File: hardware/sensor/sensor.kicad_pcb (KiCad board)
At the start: 2 copper layers, 29 x 31 mm, 56 parts, among them P1 CONN_01X05, SW1 Reset, T1 BUK9Y22, U1 LMR16006, U2 OPA376AIDCK, U3 CD74HC4046, U4 CD74HC4046, U5 Atmel_SAM_D09, X1 60V, X2 UART

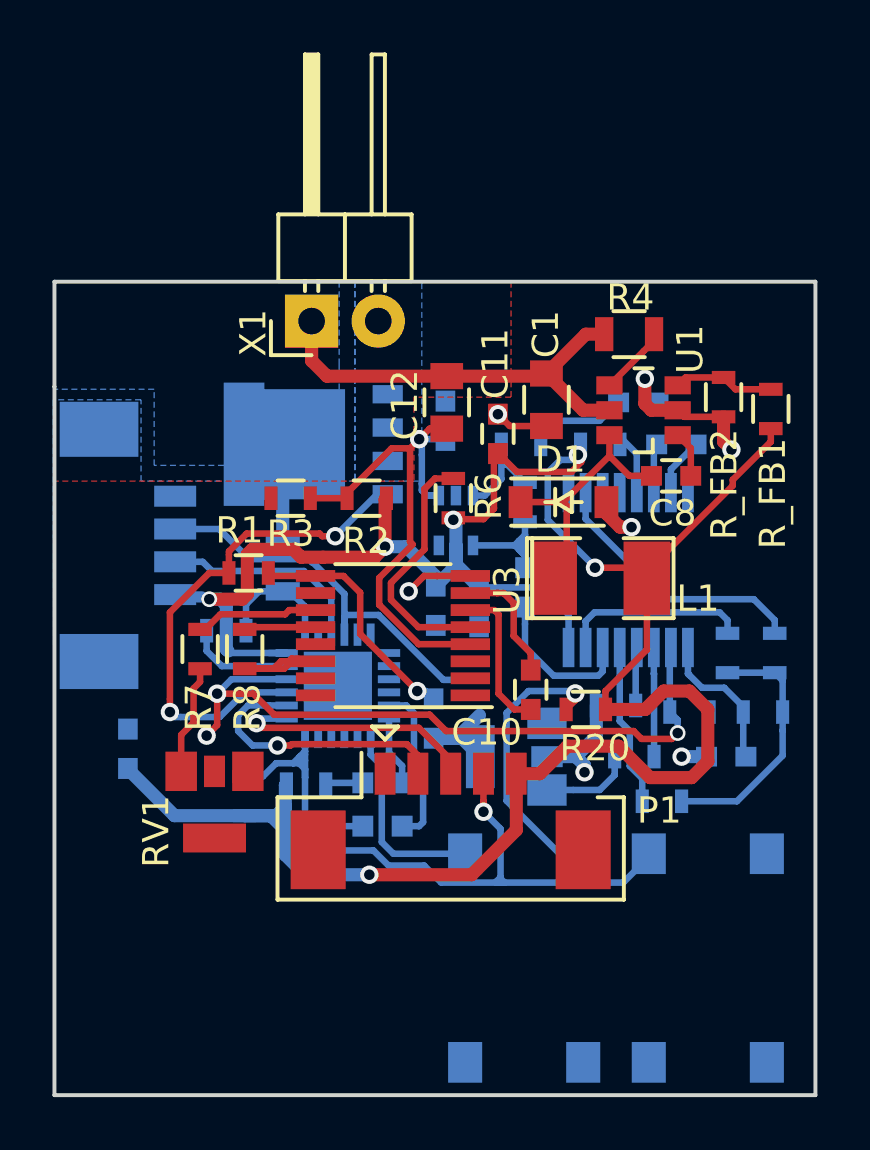
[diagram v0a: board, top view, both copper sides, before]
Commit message: Cleanup seems done
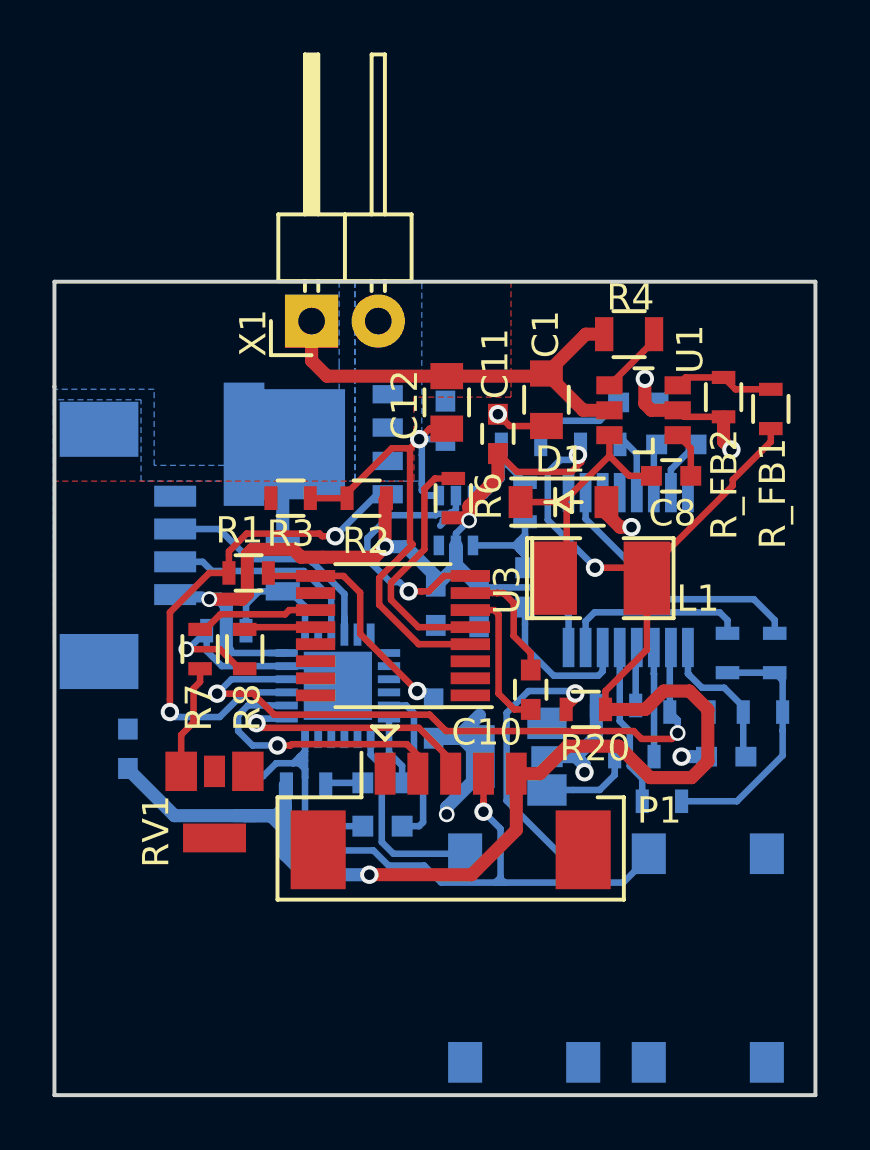
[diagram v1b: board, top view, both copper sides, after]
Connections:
- P1 pad : (no net) -> GND
- RV1 pad 4: (no net) -> GND
- RV2 pad 4: (no net) -> GND
- U3 pad 14: GND -> Net-(U3-Pad14)
- X2 pad : (no net) -> GND
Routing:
- net GND: track 30.5 -> 41.5 mm, vias 7 -> 9
- net Net-(U5-Pad4): track 15.2 -> 9.69 mm
- net /RX1_out: track 26.4 -> 24.6 mm, vias 3 -> 2
